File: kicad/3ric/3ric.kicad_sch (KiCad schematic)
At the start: 19 parts, among them U1 74LS154, U2 6502-library_65C02S-2, U8 EB6502_isc61c1024-15n

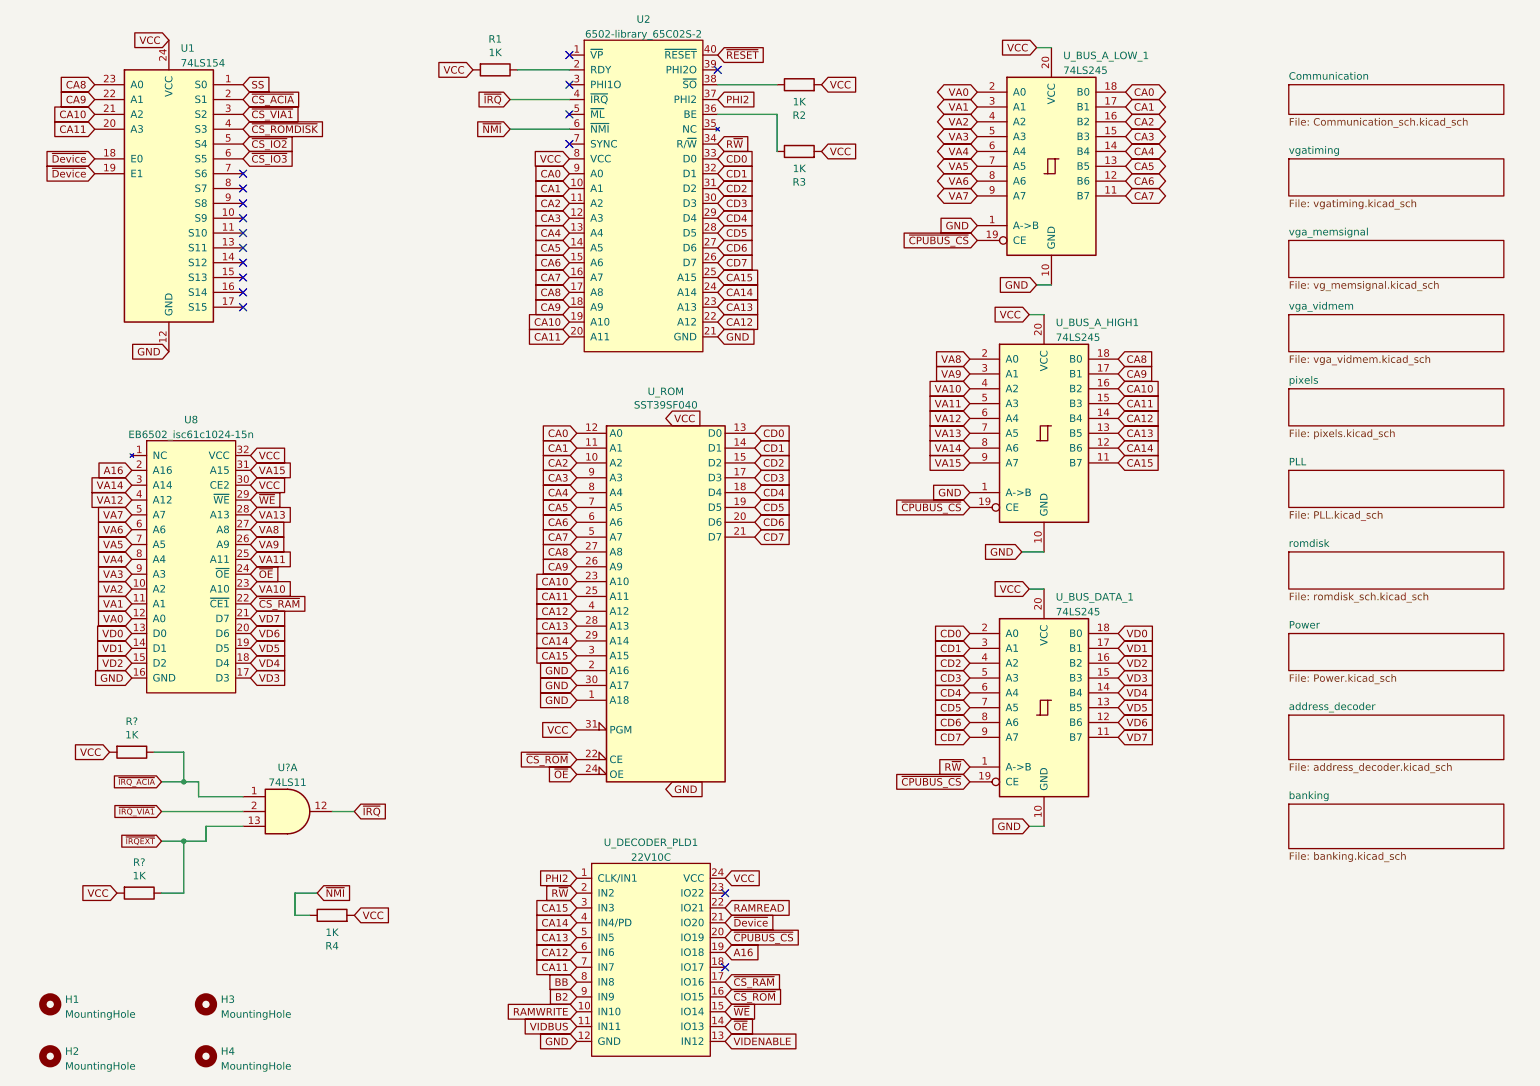
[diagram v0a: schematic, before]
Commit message: push schematic updates
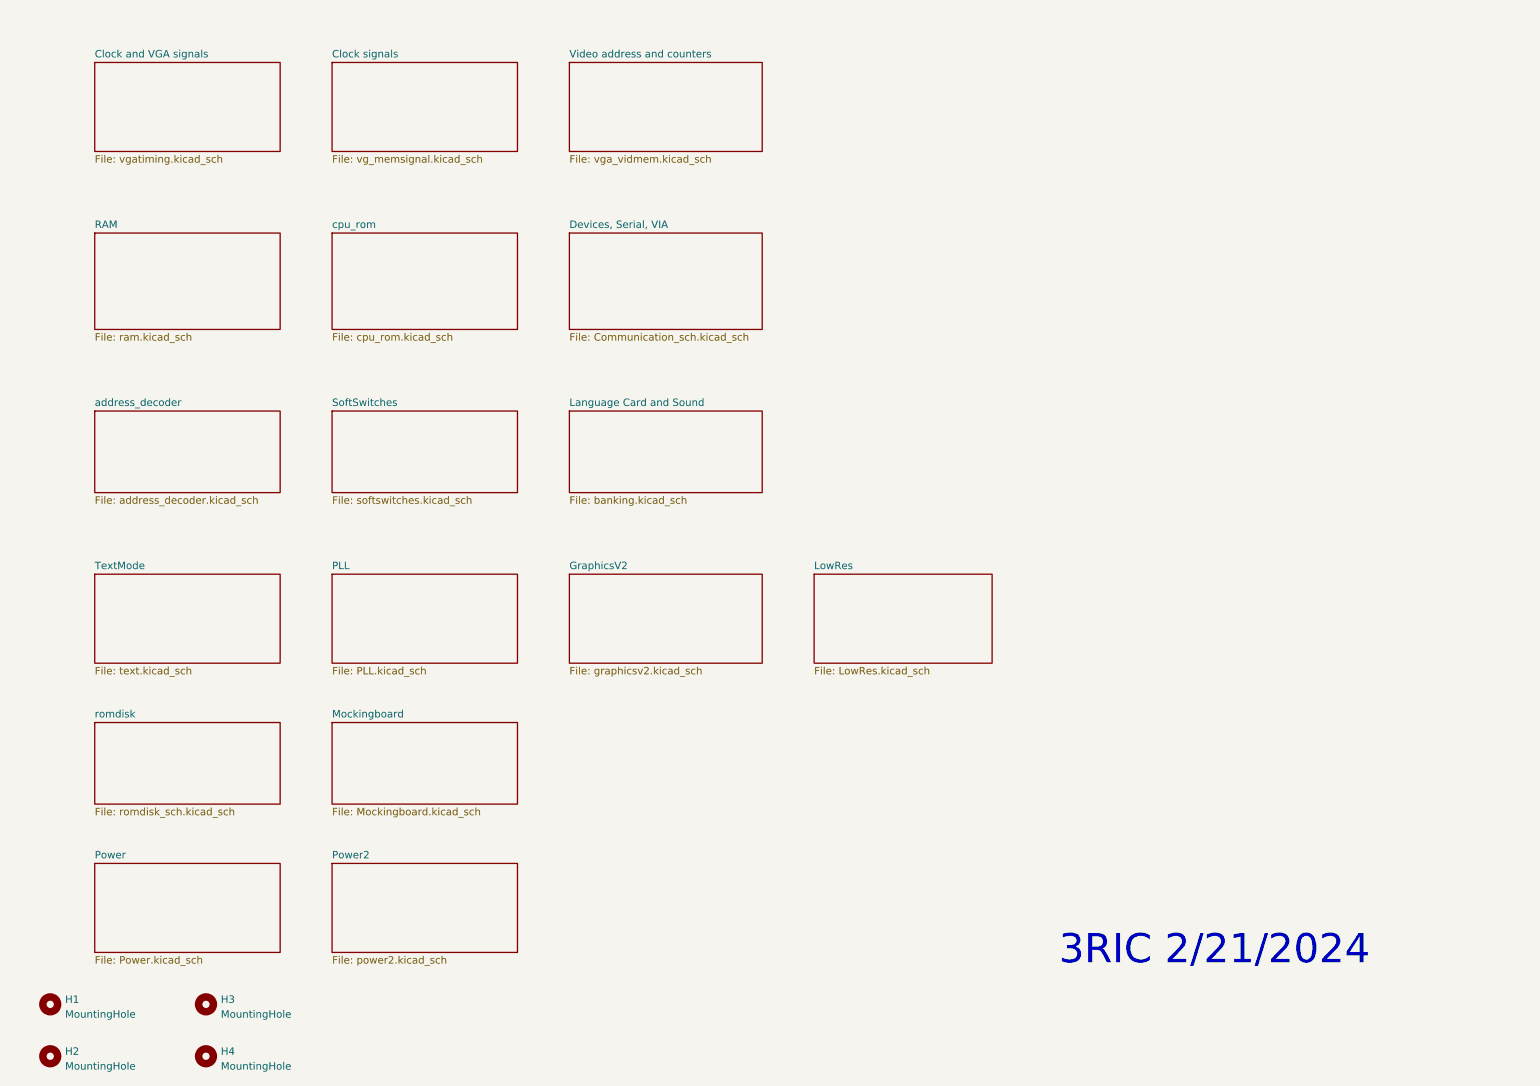
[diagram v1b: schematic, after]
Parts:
- removed R1, R2, R3, R4, R? (x2): 1K, Resistor_THT:R_Axial_DIN0207_L6.3mm_D2.5mm_P7.62mm_Horizontal, symbol Device:R
- removed U1: 74LS154, Package_DIP:DIP-24_W15.24mm_Socket, symbol 74xx:74LS154
- removed U2: 6502-library_65C02S-2, Package_DIP:DIP-40_W15.24mm_Socket, symbol EB6502-custom:6502-library_65C02S-2
- removed U8: EB6502_isc61c1024-15n, Package_DIP:DIP-32_W7.62mm, symbol EB6502-cache:EB6502_isc61c1024-15n
- removed U?: 74LS11, symbol 74xx:74LS11
- removed U_BUS_A_HIGH1, U_BUS_A_LOW_1, U_BUS_DATA_1: 74LS245, Package_DIP:DIP-20_W7.62mm_Socket, symbol 74xx:74LS245
- removed U_DECODER_PLD1: 22V10C, Package_DIP:DIP-24_W7.62mm_Socket, symbol 6502:22V10C
- removed U_ROM: SST39SF040, Package_DIP:DIP-32_W15.24mm_Socket, symbol Memory_Flash:SST39SF040
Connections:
- no-connect marks 17 -> 0
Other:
- sheet Communication renamed Devices, Serial, VIA
- sheet banking renamed Language Card and Sound
- sheet vga_memsignal renamed Clock signals
- sheet vga_vidmem renamed Video address and counters
- sheet vgatiming renamed Clock and VGA signals
- removed sheet pixels
- added sheet GraphicsV2 (graphicsv2.kicad_sch)
- added sheet LowRes (LowRes.kicad_sch)
- added sheet Mockingboard (Mockingboard.kicad_sch)
- added sheet Power2 (power2.kicad_sch)
- added sheet RAM (ram.kicad_sch)
- added sheet SoftSwitches (softswitches.kicad_sch)
- added sheet TextMode (text.kicad_sch)
- added sheet cpu_rom (cpu_rom.kicad_sch)
- note added: "3RIC 2/21/2024"
